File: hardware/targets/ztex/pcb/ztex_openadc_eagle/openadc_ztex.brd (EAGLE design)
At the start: 83.8 x 48.3 mm, 39 parts, among them CON1 DC_SOCKET5870, CON2 PWRCON, CON3 JTAG, CON6 USB-FPGA1.15, IC1 AOZ1021, IC2 AOZ1021, IC3 AOZ1094

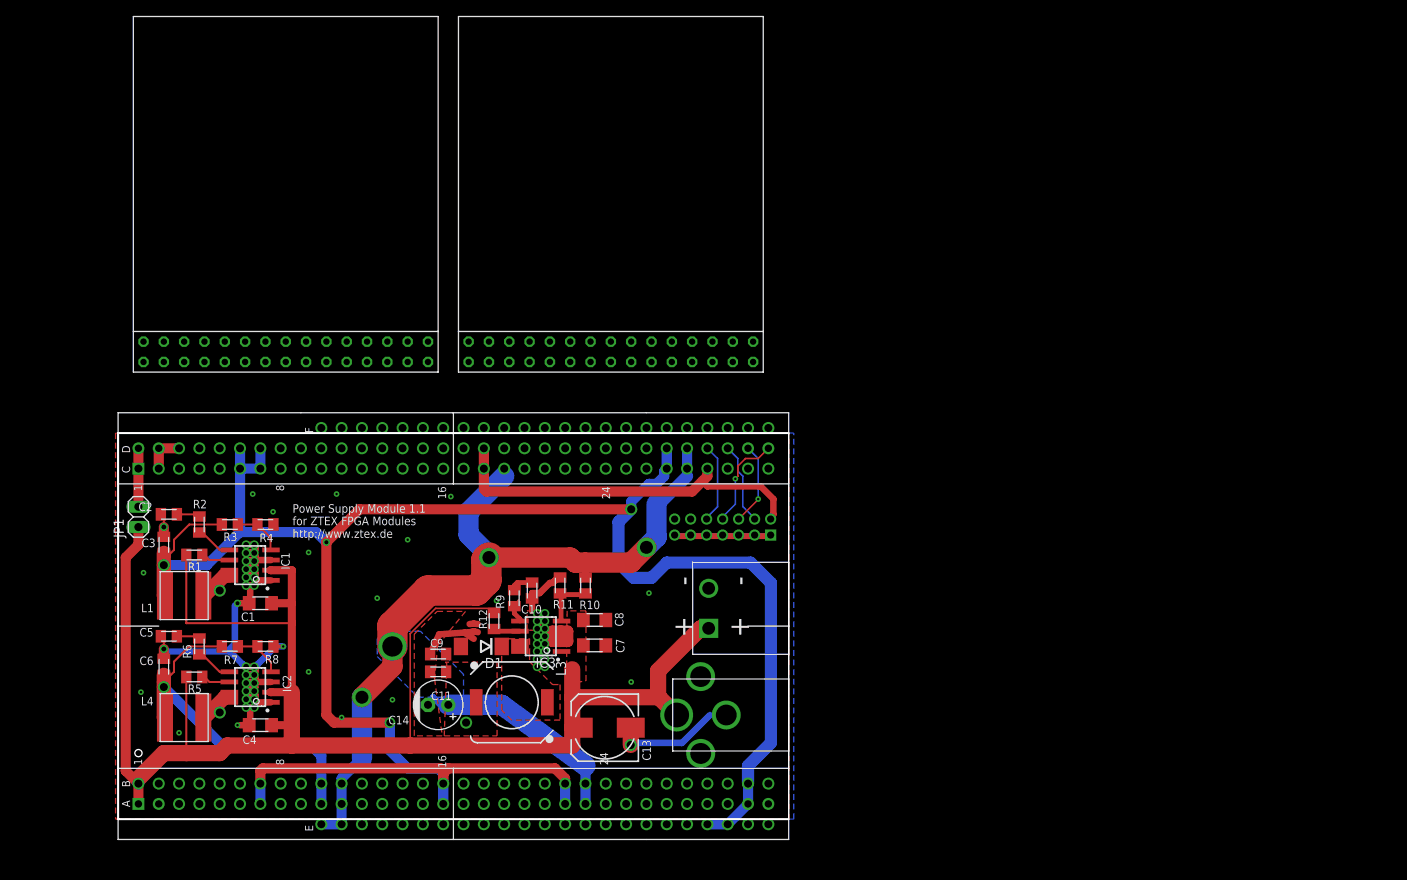
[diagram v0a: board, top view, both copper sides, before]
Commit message: More progress on ztex-pro board
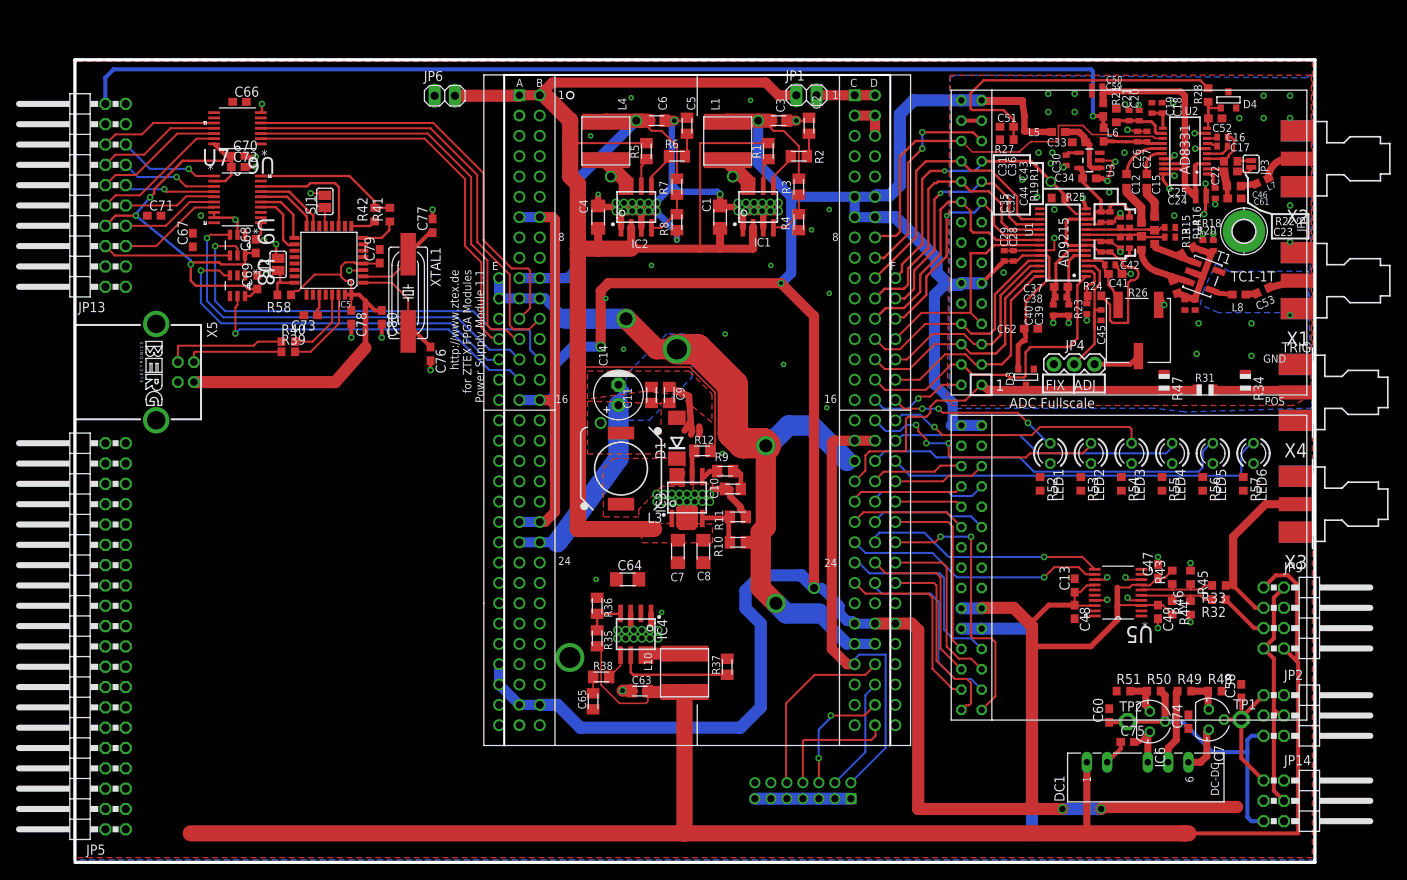
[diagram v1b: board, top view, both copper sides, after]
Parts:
- removed CON1: DC_SOCKET5870, mystuff:PWR-5870
- removed CON2: PWRCON, usb-fpga-1:PWRCON
- added C12, C15, C46: 100nF, rcl:C0603K
- added C16, C17, C19, C21, C22, C24, C26, C28, C32, C36, C38, C39, C40, C42, C45, C50, C55, C57: 100nF, rcl:C0402
- added C18, C20, C25, C27, C54, C56: 1nF, rcl:C0402
- added C23: 18nF, rcl:C0603
- added C29, C31, C35: 10nF, rcl:C0402
- added C30: 10nF, COG, rcl:C0402
- added C33, C34: 1u, rcl:C0603
- added C37, C41: 10u, rcl:C0603
- added C43, C44: (no value), rcl:C0402
- added C47, C48, C49, C66, C67, C68, C69, C70, C71, C72, C73, C76, C77, C78, C79, C80: (no value), rcl:C0603
- added C51, C52: 1uF, rcl:C0603
- added C53: (no value), rcl:C0603K
- added C58, C60, C74, C75: (no value), resistor:C0603
- added C59: 1u, rcl:C0402
- added C61: 22pF, rcl:C0603
- added C62: (no value), adc_microboard:C0603
- added C63: 22µ, myrcl:C0805K
- added C64: 10µ, myrcl:C1206
- added C65: 2n2, myrcl:C0805K
- added D3, D4: BAV99-7-F, zetex:SOT-23
- added DC1: (no value), dc-dc-converter:NMA
- added H1: MOUNT-PAD-ROUND2.8, holes:2,8-PAD
- added IC4: AOZ1021, mystuff:AOZ1021
- added IC5: AT90USB162A, adafruit:TQFP32-08
- added IC6: (no value), v-reg:337L
- added IC7: (no value), v-reg:317L
- added JP13: TARGET, pinhead:2X10/90
- added JP14, JP2: EXP-MINI, pinhead:2X03/90
- added JP3: (no value), SparkFun:SJ_2S
- added JP4: JUMPER-3PTH, SparkFun:1X03
- added JP5: (no value), pinhead:2X20/90
- added JP6: (no value), pinhead:1X02
- added JP9: PLL_INPUT, pinhead:2X04/90
- added L10: 4.7µ, myrcl:NR60
- added L2, L5, L6, L7: 120nH, SparkFun:0603
- added L8: (no value), SparkFun:0603
- added LED1, LED2, LED3, LED4, LED5, LED6: (no value), dp_devices:LED-3MM
- added R13, R14: 33R, 0.5%, adafruit:R0603
- added R15, R16: 33R, adafruit:R0603
- added R17, R18, R19, R20, R23: 1K, adafruit:R0402
- added R21: 10K, adafruit:R0603
- added R22: 274R, adafruit:R0603
- added R24: 2K, adafruit:R0603
- added R25: (no value), adafruit:R0603
- added R26: 20k, customs:3361P
- added R27, R28: 2k2, adafruit:R0603
- added R29, R30: 36R, 0.5%, adafruit:R0603
- added R31, R34, R47: (no value), adafruit:R0805
- added R32, R33, R39, R40, R41, R42, R43, R44, R45, R46, R48, R49, R50, R51, R52, R53, R54, R55, R56, R57, R58: (no value), resistor:R0603
- added R35, R36: ?, myrcl:R0805K
- added R37, R38: 7K5, myrcl:R0805K
- added SJ1, SJ2: (no value), jumper:SJ
- added T1: TC1-1T, customs:AT224-1A
- added TP1, TP2: TPSQPAD1-13, testpad:P1-13
- added U1: AD9215BRUZ, customs:TSSOP28
- added U2: AD8331, customs:QSOP20
- added U3: LP3985IM5-3.0, SparkFun:SOT23-5
- added U5: CDCE906PW, Texas Instruments_By_element14_Batch_1:SOP65P640X120-20N
- added U6: TXB0104PWR, Texas Instruments_By_element14_Batch_1:SOP65P640X120-14N
- added U7: TXB0108PWR, Texas Instruments_By_element14_Batch_1:SOP65P640X120-20N
- added U8, U9: SN74LVC1T45DBVT, Texas Instruments_By_element14_Batch_1:SOT95P280X145-6N
- added X1, X2, X3, X4: SMA-142-0711-821/826, con-coax:J502-ND-142-0711-821/826
- added X5: PN61729-S, con-berg:PN61729-S
- added XTAL1: (no value), dp_devices:HC-49U
- C13: value 220µ -> (none); device myrcl:153CLV-0810 -> rcl:C0603
- moved CON6 104.8 mm to (53.7, 98.1), turned to 270 degrees
- moved JP1 98.7 mm to (91.4, 95.6), turned to 0 degrees
- moved C2 93.6 mm to (91.8, 91.8), turned to 270 degrees
- moved C3 93.4 mm to (87.9, 92.4), turned to 180 degrees
- moved C6 91.9 mm to (72.7, 92.4), turned to 180 degrees
- moved C5 90.9 mm to (76.5, 91.8), turned to 270 degrees
- moved L4 89.3 mm to (66.4, 89.9), turned to 90 degrees
- moved L1 88.6 mm to (81.6, 89.9), turned to 90 degrees
- moved R2 87.9 mm to (90.5, 87.9), turned to 180 degrees
- moved U$3 87.9 mm to (113.3, 77.2), turned to 180 degrees
- moved R1 87.7 mm to (86.7, 88.6), turned to 90 degrees
- moved R5 86.7 mm to (71.4, 88.6), turned to 90 degrees
- moved R6 85.5 mm to (75.2, 87.9), turned to 180 degrees
- moved R3 82.7 mm to (90.5, 84.1), turned to 90 degrees
- moved R7 80.2 mm to (75.2, 84.1), turned to 90 degrees
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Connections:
- new net +5V: C63.2, DC1.1, JP13.1, JP13.20, JP9.1, JP9.8, L10.P$2, L2.1, L6.1, R35.2
- new net +5V/2: C66.1, C78.1, C79.1, C80.1, IC5.31, IC5.32, IC5.4, JP6.1, R58.1, U7.19, X5.1
- new net +9V: C58.1, IC7.2, JP14.1, JP2.1, R48.2, TP1.TP
- new net -9V: C60.1, IC6.OUT, JP14.5, JP2.5, R50.2, TP2.TP
- new net ADC_VCC: C31.1, C32.1, C34.1, C35.1, C36.1, R17.2, R19.1, R24.2, U1.12, U1.7, U3.5
- new net AGND: C45.2, C62.2, D3.3
- new net CLK_PLL0: CON6.D23, U5.11
- new net CLK_PLL1: CON6.C23, U5.12
- new net DGND: X3.G@1, X3.G@2, X3.G@3, X3.G@4
- new net HS1: CON6.E14, U8.3
- new net HS1DIR: CON6.A15, U8.5
- new net HS2: CON6.A14, U9.3
- new net HS2DIR: CON6.B14, U9.5
- new net LED1: CON6.F16, LED1.A
- new net LED2: CON6.D17, LED2.A
- new net LED3: CON6.F17, LED3.A
- new net LED4: CON6.F18, LED4.A
- new net LED5: CON6.D19, LED5.A
- new net LED6: CON6.F19, LED6.A
- new net N$100: JP13.6, U9.4
- new net N$101: JP13.4, U8.4
- new net N$102: IC5.29, R40.2
- new net N$103: R40.1, X5.3
- new net N$104: R39.1, X5.2
- new net N$105: IC5.9, R42.1
- new net N$106: C73.1, IC5.27
- new net N$107: IC5.8, R41.1
- new net N$108: IC6.ADJ, R50.1, R51.2
- new net N$109: IC7.1, R48.1, R49.2
- new net N$11: C12.1, U2.15
- new net N$110: LED1.K, R52.1
- new net N$111: LED2.K, R53.1
- new net N$112: LED3.K, R54.1
- new net N$113: LED4.K, R55.1
- new net N$114: LED5.K, R56.1
- new net N$115: LED6.K, R57.1
- new net N$116: C76.1, IC5.1, XTAL1.2
- new net N$117: C77.1, IC5.2, XTAL1.1
- new net N$118: JP9.3, R33.1, X3.1
- new net N$12: C17.2, U2.5
- new net N$122: IC5.13, SJ1.1
- new net N$123: IC5.24, R58.2, SJ2.1
- new net N$16: C17.1, U2.7
- new net N$18: C16.2, U2.8
- new net N$19: C16.1, R22.2, U2.4
- new net N$21: C18.1, C19.1, U2.11
- new net N$22: C20.1, C21.1, R21.1, U2.12
- new net N$27: C22.2, U2.1
- new net N$28: C23.1, C46.1, C61.1, U2.2
- new net N$29: C23.2, JP3.1
- new net N$30: JP3.2, R22.1
- new net N$31: C26.1, C27.1, L6.2, U2.14
- new net N$55: C30.2, U3.4
- new net N$56: C33.1, L5.2, U3.1, U3.3
- new net N$57: C37.1, C38.1, C39.2, U1.5
- new net N$58: C37.2, C38.2, C40.2, U1.6
- new net N$59: C41.2, C42.2, R26.3, U1.4
- new net N$6: C44.1, R13.1, R15.2, R19.2, R20.2, U1.9
- new net N$60: C45.1, JP4.2, U1.3
- new net N$61: R23.1, R24.1, U1.2
- new net N$62: C43.1, R14.1, R16.2, R17.1, R18.1, U1.10
- new net N$63: JP4.1, R26.2
- new net N$64: L7.1, X2.1
- new net N$65: JP9.5, R32.1
- new net N$67: C51.1, R27.2, R28.1
- new net N$68: C52.1, D4.3, R28.2, U2.10
- new net N$69: C24.1, C25.1, C50.1, C59.2, L2.2, U2.18, U2.19, U2.3
- new net N$7: C12.2, R15.1
- new net N$70: R14.2, R30.1, T1.3
- new net N$71: C53.2, X1.1
- new net N$72: C53.1, L8.1
- new net N$73: L8.2, T1.6
- new net N$75: R13.2, R29.2, T1.1
- new net N$76: C54.1, C55.1, C56.2, C57.2, R29.1, R30.2, T1.2
- new net N$77: R33.2, R43.1, R45.2, U5.6
- new net N$78: C46.2, L7.2
- new net N$79: IC4.LX, L10.P$1
- new net N$8: C15.2, R16.1
- new net N$80: R31.1, R34.2, X4.1
- new net N$81: R32.2, R44.1, R46.2, U5.5
- new net N$82: C74.1, DC1.6, IC7.3
- new net N$83: IC4.FB, R35.1, R36.2
- new net N$84: IC4.EN, R37.1
- new net N$85: C65.2, R38.1
- new net N$86: IC4.COMP, R38.2
- new net N$87: JP13.5, U7.7
- new net N$88: IC5.30, R39.2
- new net N$89: JP13.16, U6.10
- new net N$9: C15.1, U2.16
- new net N$90: JP13.14, U6.11
- new net N$91: JP13.12, U6.12
- new net N$92: JP13.10, U6.13
- new net N$93: C68.1, C69.1, C70.1, C71.1, C72.1, JP13.8, U6.14, U7.2, U8.6, U9.6
- new net N$94: JP13.7, U7.6
- new net N$95: JP13.9, U7.5
- new net N$96: JP13.11, U7.4
- new net N$97: JP13.13, U7.3
- new net N$98: JP13.15, U7.1
- new net N$99: C75.2, DC1.4, IC6.IN
- new net PRG_MISO: IC5.17, U7.15
- new net PRG_MOSI: IC5.16, U7.16
- new net PRG_PDIC: IC5.11, U7.18
- new net PRG_PDID: R41.2, R42.2, U7.20
- new net PRG_RST: IC5.18, U7.14
- new net PRG_SCK: IC5.15, U7.17
- new net TARGET1: CON6.E13, U6.2
- new net TARGET2: CON6.A13, U6.3
- new net TARGET3: CON6.B12, U6.4
- new net TARGET4: CON6.A12, U6.5
- new net VCCIO: U6.1, U8.1, U9.1
- net +3V3: now also C13.1, C28.1, C29.1, C47.1, C48.1, C49.1, C62.1, C67.1, D3.2, JP13.18, JP13.3, JP14.4, JP2.4, JP9.2, JP9.7, L5.1, R43.2, R44.2, U$3.11, U$3.12, U$3.29, U$3.30, U$5.11, U$5.12, U$5.29, U$5.30, U1.24, U5.14, U5.18, U5.3, U5.7
- net GND: now also C13.2, C18.2, C19.2, C20.2, C21.2, C22.1, C24.2, C25.2, C26.2, C27.2, C28.2, C29.2, C30.1, C31.2, C32.2, C33.2, C34.2, C35.2, C36.2, C39.1, C40.1, C41.1, C42.1, C43.2, C44.2, C47.2, C48.2, C49.2, C50.2, C51.2, C52.2, C54.2, C55.2, C56.1, C57.1, C58.2, C59.1, C60.2, C61.2, C63.1, C64.1, C65.1, C66.2, C67.2, C68.2, C69.2, C70.2, C71.2, C72.2, C73.2, C74.2, C75.1, C76.2, C77.2, C78.2, C79.2, C80.2, D4.2, DC1.2, DC1.5, IC4.AGND, IC4.PGND, IC5.28, IC5.3, JP13.17, JP13.19, JP13.2, JP14.2, JP14.6, JP2.2, JP2.6, JP4.3, JP9.4, JP9.6, R18.2, R20.1, R21.2, R23.2, R25.1, R26.1, R34.1, R36.1, R45.1, R46.1, R47.1, R49.1, R51.1, R52.2, R53.2, R54.2, R55.2, R56.2, R57.2, SJ1.2, SJ2.2, T1.4, U$3.10, U$3.27, U$3.28, U$3.9, U$5.10, U$5.27, U$5.28, U$5.9, U1.11, U1.14, U1.23, U1.8, U2.17, U2.20, U2.6, U2.9, U3.2, U5.13, U5.17, U5.4, U5.8, U6.7, U7.11, U7.8, U7.9, U8.2, U9.2, X1.G@1, X1.G@2, X1.G@3, X1.G@4, X2.G@1, X2.G@2, X2.G@3, X2.G@4, X4.G@1, X4.G@2, X4.G@3, X4.G@4, X5.4, X5.S1, X5.S2; no longer C13.-, CON1.3, CON2.-
- net OA_ADC0: now also U1.17
- net OA_ADC1: now also U1.18
- net OA_ADC2: now also U1.19
- net OA_ADC3: now also U1.20
- net OA_ADC4: now also U1.21
- net OA_ADC5: now also U1.22
- net OA_ADC6: now also U1.25
- net OA_ADC7: now also U1.26
- net OA_ADC8: now also U1.27
- net OA_ADC9: now also U1.28
- net OA_ADCOR: now also U1.1
- net OA_CLKADC: now also R25.2, U1.13
- net OA_CLKIN: now also D3.1, R31.2, R47.2
- net OA_GAIN: now also R27.1
- net OA_HILO: now also U2.13
- net VIN: now also C64.2, IC4.VIN, JP6.2, R37.2; no longer C13.+, CON1.1, CON2.+
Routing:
- net +5V: track 0.00 -> 358.7 mm, vias 0 -> 1
- net +3V3: track 261.6 -> 541.4 mm, vias 4 -> 6
- net GND: track 138.6 -> 261.1 mm, vias 62 -> 148
- net N$93: track 0.00 -> 58.8 mm, vias 0 -> 3
- net HS2DIR: track 0.00 -> 55.6 mm, vias 0 -> 1
- net TARGET3: track 0.00 -> 54.5 mm
- net +5V/2: track 0.00 -> 54.4 mm
- net HS2: track 0.00 -> 53.0 mm, vias 0 -> 1
- net OA_CLKIN: track 0.00 -> 52.8 mm
- net TARGET4: track 0.00 -> 52.8 mm
- net TARGET2: track 0.00 -> 52.6 mm
- net OA_HILO: track 0.00 -> 50.2 mm
- net TARGET1: track 0.00 -> 49.8 mm
- net LED6: track 0.00 -> 48.9 mm
- net HS1: track 0.00 -> 48.2 mm, vias 0 -> 1
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- added copper zone on layer 16, net N$74
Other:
- board size 83.8 x 48.3 mm -> 155 x 100.3 mm
- board text added: "1"
- board text added: "AD8331"
- board text added: "AD9215"
- board text added: "ADC Fullscale"
- board text added: "ADJ"
- board text added: "FIX"
- board text added: "GND"
- board text added: "JP3"
- board text added: "POS"
- board text added: "TC1-1T"
- board text added: "TRIG"
